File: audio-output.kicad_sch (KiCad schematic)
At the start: 12 parts, among them J2 AudioJack3_Switch, U4 LM386

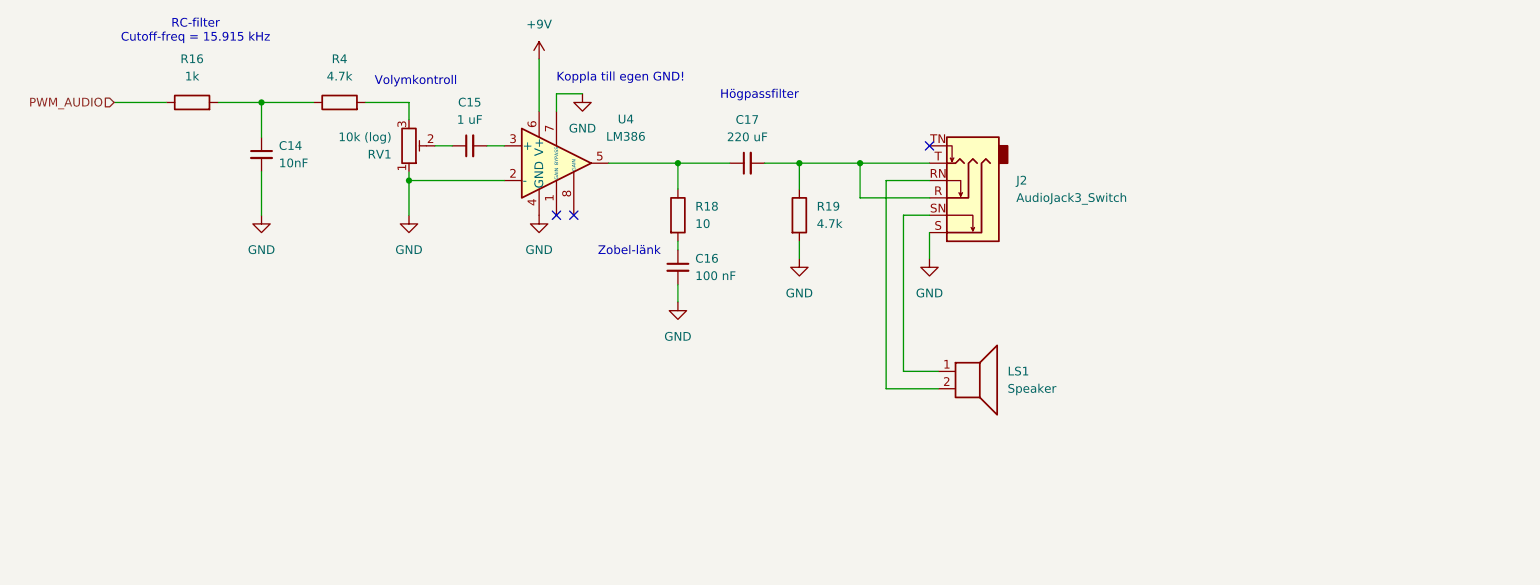
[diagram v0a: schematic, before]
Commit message: Update kicad to rev 0.1
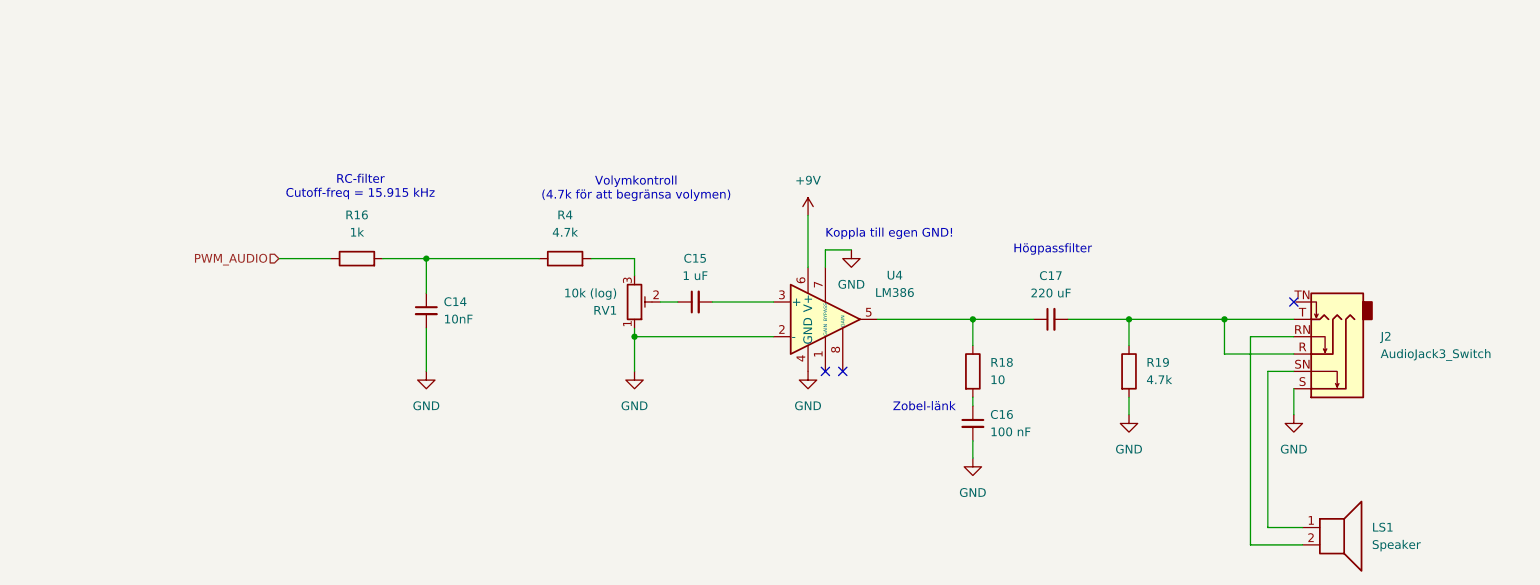
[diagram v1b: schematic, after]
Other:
- note added: "Volymkontroll (4.7k för att begränsa volymen)"
- note removed: "Volymkontroll"
- moved on the sheet: C14, C15, C16, C17, J2, LS1, R16, R18, R19, R4, RV1, U4
